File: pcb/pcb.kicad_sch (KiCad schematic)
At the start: 81 parts, among them J1 USB_B_Micro, J2 battery, J3 SD_Card, J4 swd, J5 speakers, SW1 RotaryEncoder, SW2 next, SW3 play, U1 TP4056, U2 LM358, U3 ME2149, U4 PCM1754, U5 CC2640, U6 LM4810, U7 LM358, Y1 24M

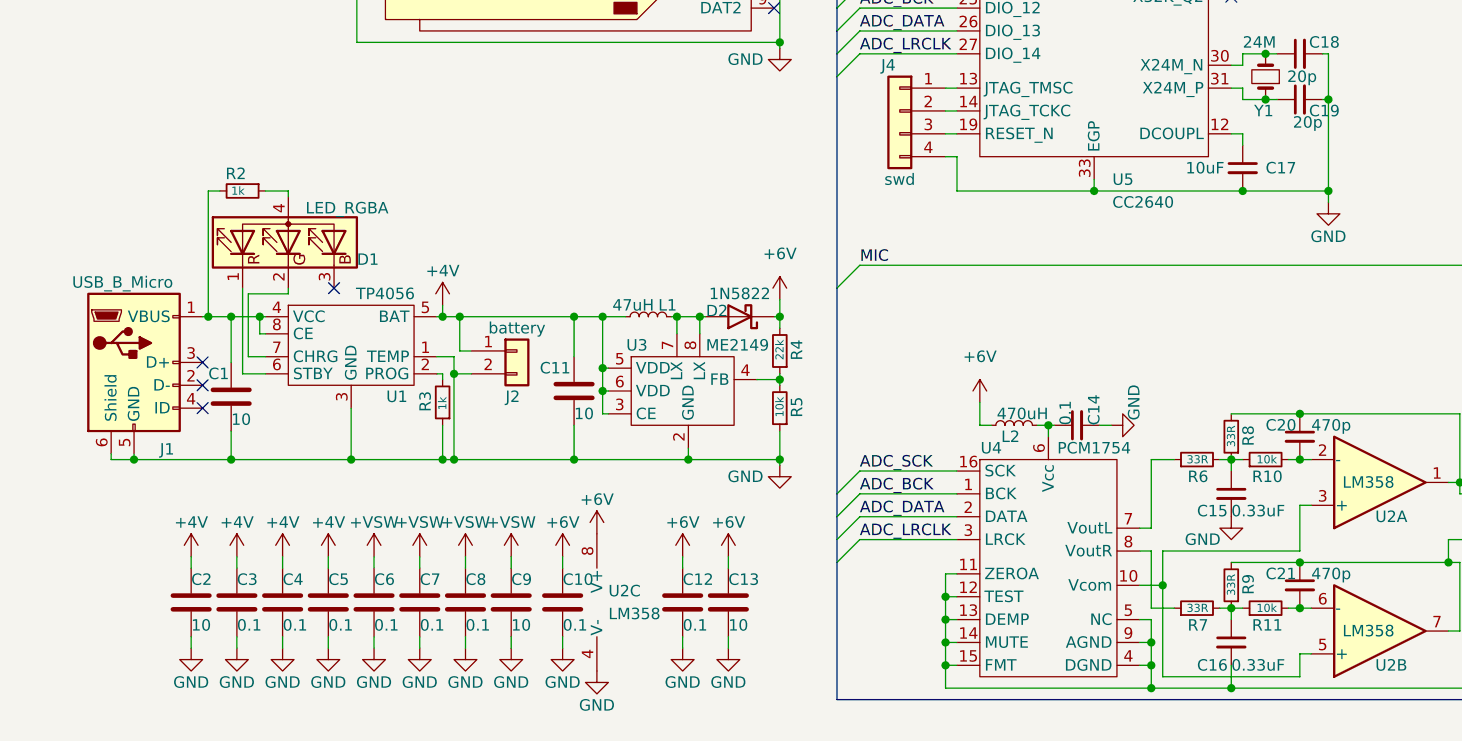
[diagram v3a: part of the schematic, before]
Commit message: pcb block wiev
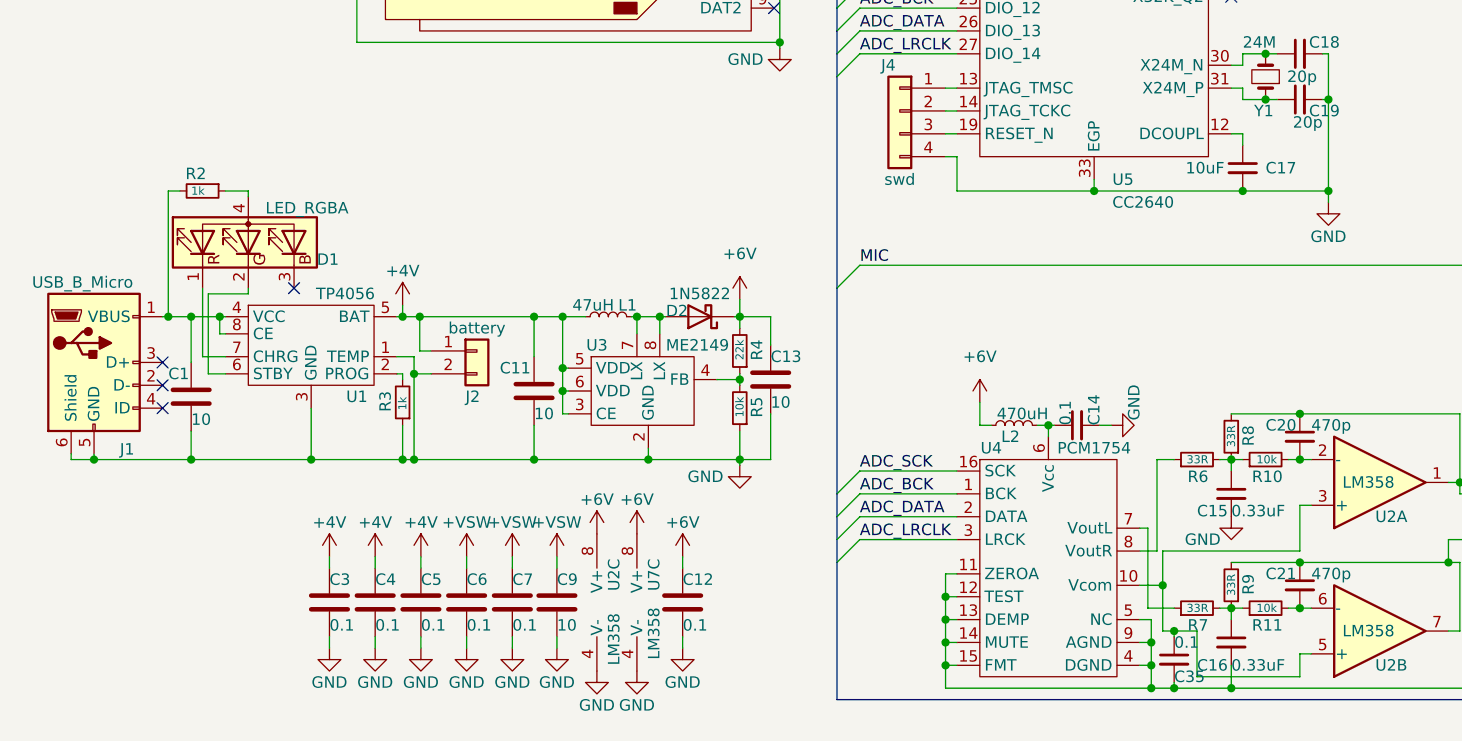
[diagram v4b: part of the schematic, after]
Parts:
- removed C10, C8: 0.1, Capacitor_SMD:C_0402_1005Metric, symbol Device:C
- removed C2: 10, Capacitor_SMD:C_0805_2012Metric, symbol Device:C
- added C35: 0.1, Capacitor_SMD:C_0402_1005Metric, symbol Device:C_Small
- added unit 3 of U7
- L1: footprint Inductor_SMD:L_0603_1608Metric -> Inductor_SMD:L_1206_3216Metric
- U3: footprint Package_SO:SOIC-8-N7_3.9x4.9mm_P1.27mm -> Package_SO:SOP-8_3.9x4.9mm_P1.27mm
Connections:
- net +6V: now also U7.8 (V+)
- net GND: now also C35.2, U7.4 (V-)
- net at R7.1: now also U4.7 (VoutL); no longer U4.8 (VoutR)
- net at U2.3 (+), U2.5 (+), U4.10 (Vcom): now also C35.1
- net at R6.1: now also U4.8 (VoutR); no longer U4.7 (VoutL)
- net at U1.6 (STBY): now also D1.2 (GK); no longer D1.1 (RK)
- net at U1.7 (CHRG): now also D1.1 (RK); no longer D1.2 (GK)
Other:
- moved on the sheet: C1, C11, C13, C3, C4, C5, C6, C7, C9, D1, D2, J1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
